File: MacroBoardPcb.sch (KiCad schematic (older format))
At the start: 32 parts, among them SW1 SW_Push, SW2 Rotary_Encoder_Switch, U1 ATmega32U4-AU, Y1 16MHz

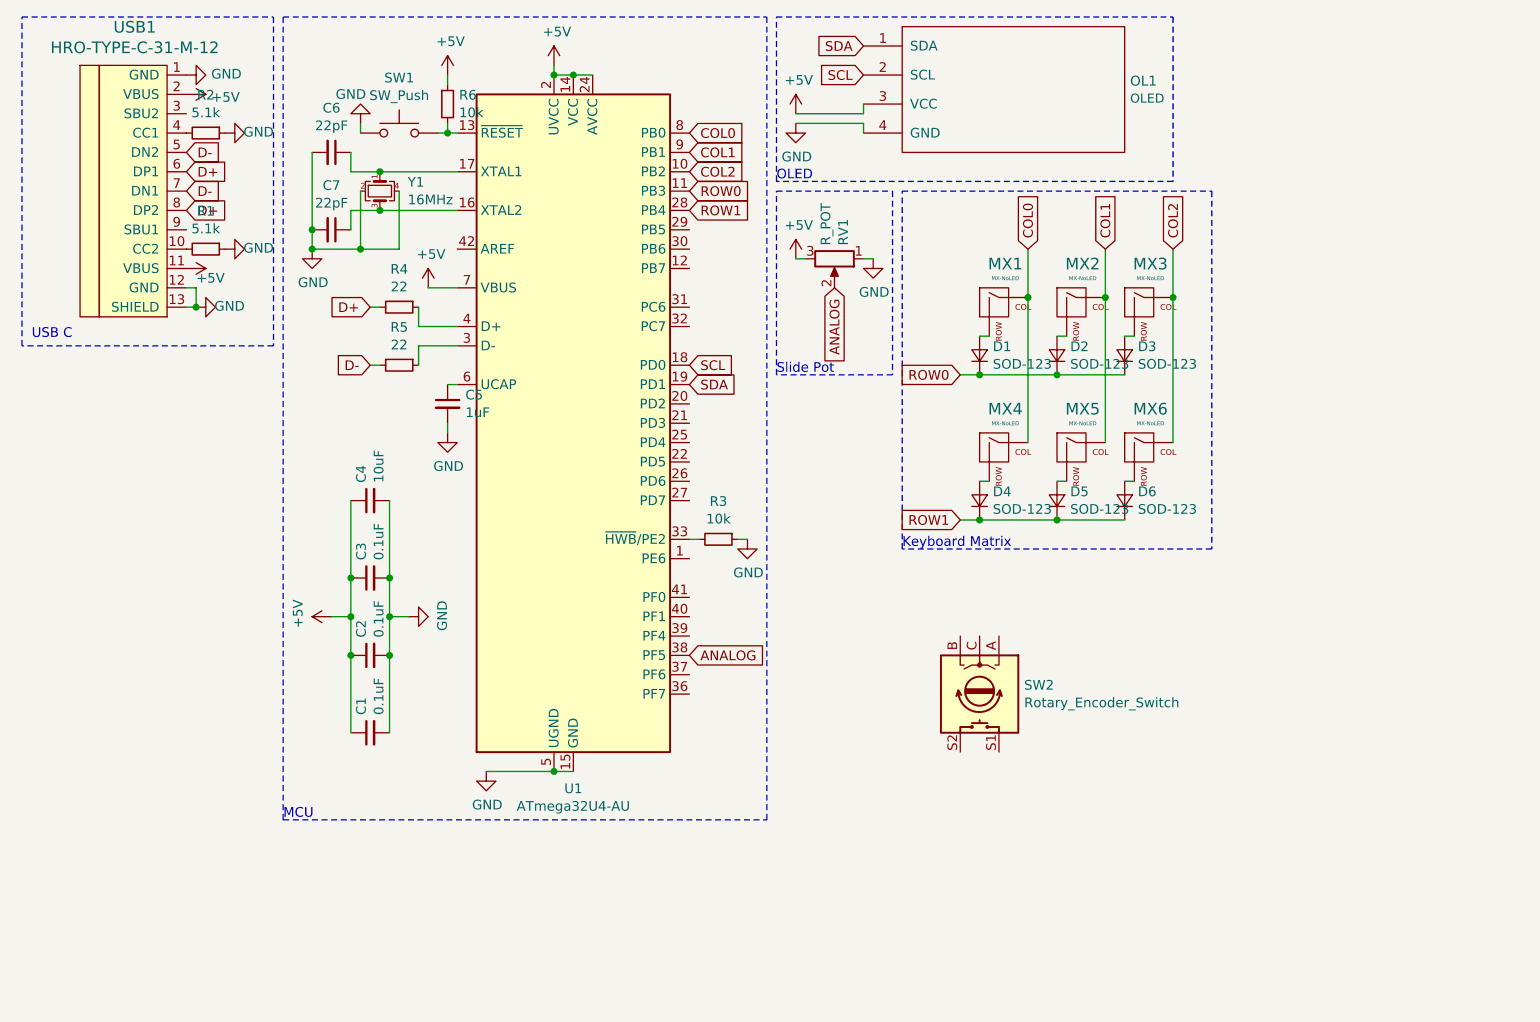
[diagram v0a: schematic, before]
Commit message: finished schematics
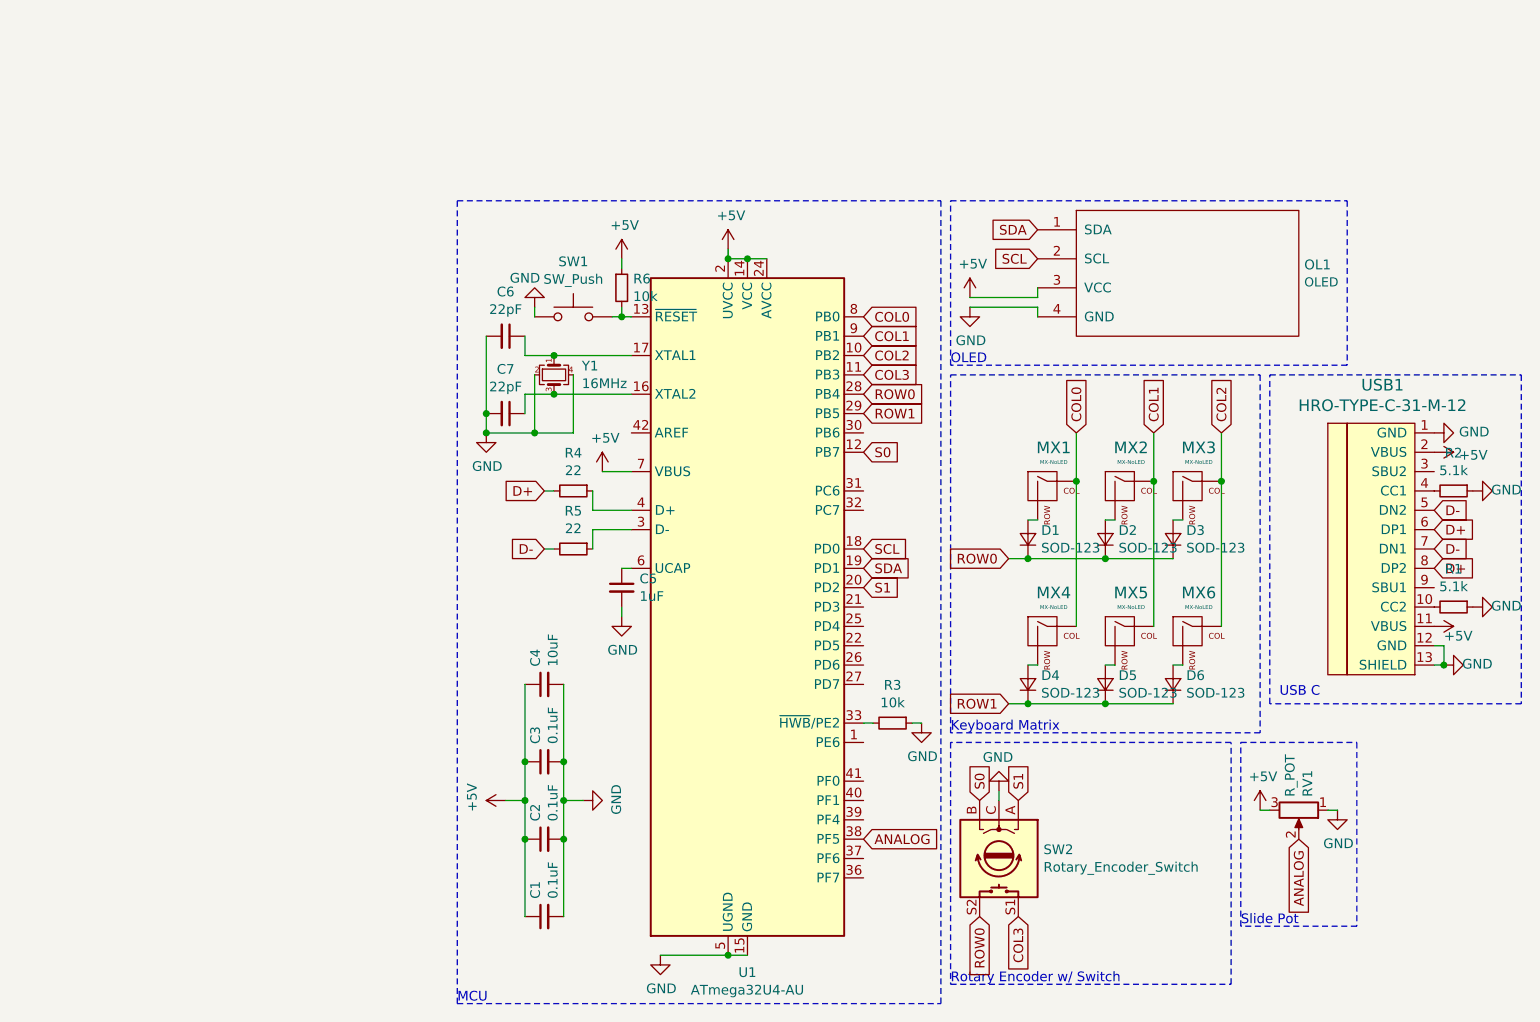
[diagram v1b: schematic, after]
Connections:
- net GND: now also SW2.C
- net ROW0: now also SW2.S2, U1.28 (PB4); no longer U1.11 (PB3)
- net ROW1: now also U1.29 (PB5); no longer U1.28 (PB4)
- net S0: now reaches U1.12 (PB7)
- net S0: now also SW2.B
- net S1: now reaches U1.20 (PD2)
- net S1: now also SW2.A
- net COL3: now reaches SW2.S1
- net COL3: now also U1.11 (PB3)
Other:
- note added: "Rotary Encoder w/ Switch\n"
- moved on the sheet: C1, C2, C3, C4, C5, C6, C7, D1, D2, D3, D4, D5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
